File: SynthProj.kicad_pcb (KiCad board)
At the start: 4 copper layers, 304.8 x 110 mm, 649 parts, among them J1 PWM IN, J10 Mixer Ext In, J11 S&H_Out, J12 LFOA_Out, J13 Gate, J14 1V/Oct CV, J18 Ext In, J2 Exp CV In, J20 ADEG1_OUT, J21 ADEG2_OUT, J25 Master Output, J26 RP2040_A_in, J27 RP2040_B_in, J28 RP2040_C_in, J3 Lin CV In, J30 Echo_DV, J31 Echo_Repeat, J32 Echo_CV_In, J33 Echo_ExtIn, J34 ECHO_OUT, J35 RP2040_A_out, J36 RP2040_B_out, J37 locked, J38 locked, J39 Noise Out, J4 Sync, J40 Conn_01x02, J41 DIN-504D-M5, J42 USB_B, J43 Conn_01x02, J44 Jack-DC, J5 Conn_01x18, J6 S&H_In, J7 Lin CV In, J8 Exp CV In, J9 PWM IN, Q1 MMBF4393LT1G, Q10 MMBT3904-7-F, Q11 MMBT3904-7-F, Q12 MMBF4391LT1G, Q13 MMBT3904-7-F, Q14 MMBT3904-7-F, Q15 MMBT3906LT1G, Q16 MMBF5457, Q17 MMBF5457, Q18 MMBT3906LT1G, Q19 MMBF5457, Q2 MMBT3904-7-F, Q21 MMBT3904-7-F, Q22 MMBT3904-7-F, Q23 MMBT3906LT1G, Q24 MMBT3906LT1G, Q3 MMBT3906LT1G, Q4 MMBT3904-7-F, Q5 MMBT3906LT1G, Q6 MMBF4393LT1G, Q7 MMBT3904-7-F, Q8 MMBT3904-7-F, Q9 MMBF4391LT1G, SW1 SW_SPST, SW10 SW_SPDT, SW11 SW_SPDT, SW12 SMTS-103-A1-T0, SW13 SW_Push_DPDT, SW14 SW_SPST, SW15 SW_Push, SW16 SW_SPST, SW17 SW_SPDT, SW18 SW_SPDT, SW19 SW_Push, SW2 SW_SPDT, SW20 SW_DPST, SW21 SW_DPST, SW22 SW_SPST, SW23 SW_SPST, SW3 SW_SPDT, SW4 SW_SPDT, SW5 SW_DPDT_x2, SW56 SW_Push, SW58 SW_Push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

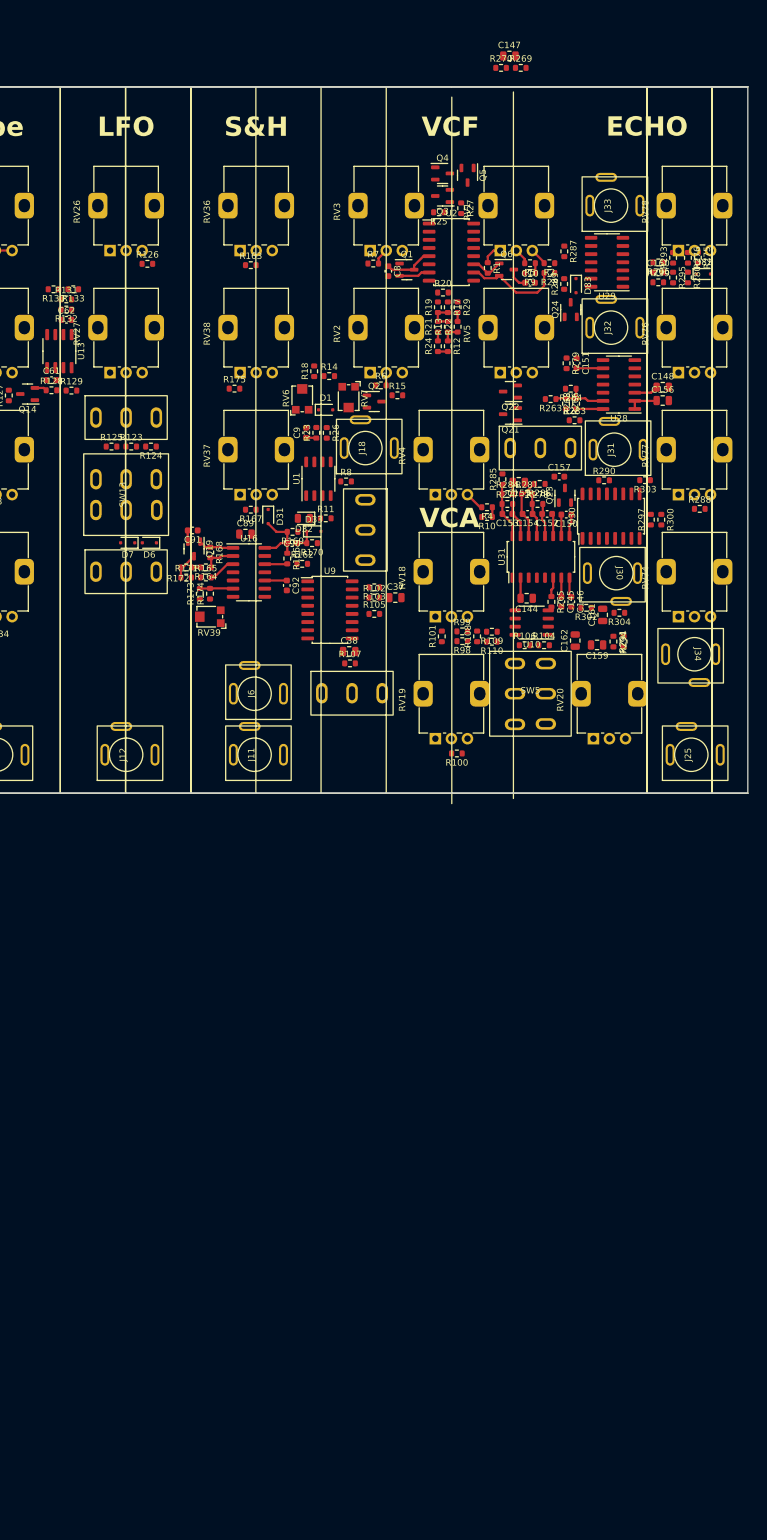
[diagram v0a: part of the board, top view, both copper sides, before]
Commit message: work
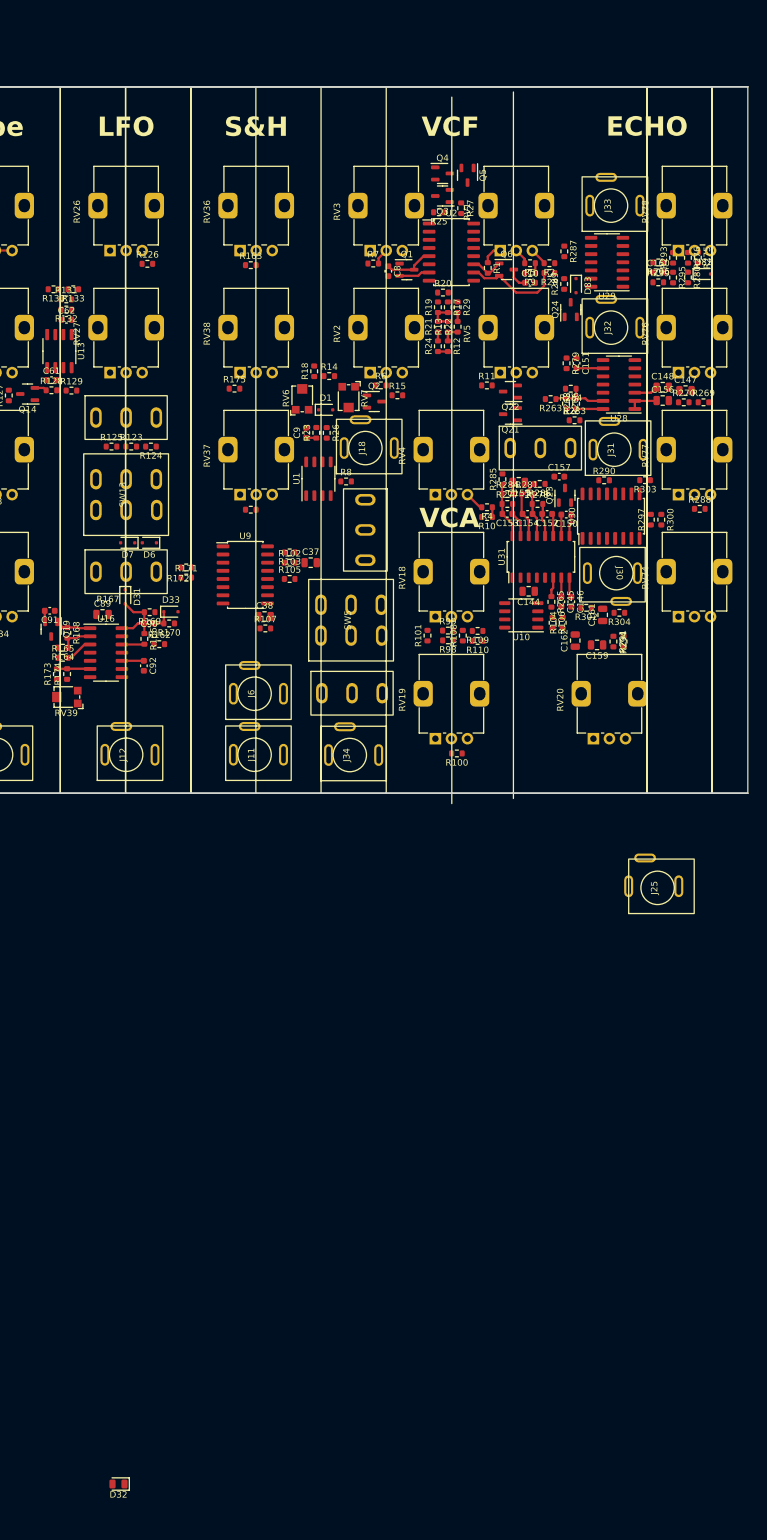
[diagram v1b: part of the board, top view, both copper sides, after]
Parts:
- moved D32 153.1 mm to (301.8, 354.6)
- moved R270 59.3 mm to (389.8, 186.1)
- moved R269 59.3 mm to (392.9, 186.1)
- moved C147 58.9 mm to (390.1, 184.3)
- moved J34 55.9 mm to (337.8, 241.0), turned to 90 degrees
- moved R11 32.5 mm to (359.2, 183.5)
- moved SW5 30.2 mm to (338.0, 220.1), turned to 90 degrees
- moved C89 25.5 mm to (299.3, 219.2)
- moved C90 25.5 mm to (306.6, 220.6)
- moved C92 25.5 mm to (305.8, 227.1)
- moved D33 25.5 mm to (310.0, 218.7)
- moved R169 25.5 mm to (306.7, 218.8)
- moved RV39 25.5 mm to (293.7, 232.0)
- moved C91 25.5 mm to (291.1, 218.6)
- moved D31 25.5 mm to (302.9, 216.4)
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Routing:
- net Net-(Q19-G): track 4.34 -> 0.00 mm
- net Net-(U31-REF): track 3.20 -> 0.00 mm
- net -12V: track 4.61 -> 3.20 mm
